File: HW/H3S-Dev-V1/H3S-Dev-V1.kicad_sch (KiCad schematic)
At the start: 38 parts, among them J1 USB_C_Receptacle_USB2.0_16P, J2 Conn_01x02_Socket, J3 Conn_Coaxial, Q1 DMP3099L, SW1 SW_Push, U1 Ai-Thinker-Ra-01, U2 LTC4054ES5-4.2, U3 USBLC6-2SC6, U4 ESP32-S3-WROOM-1, U5 SY8089AAAC, U6 L96-M33

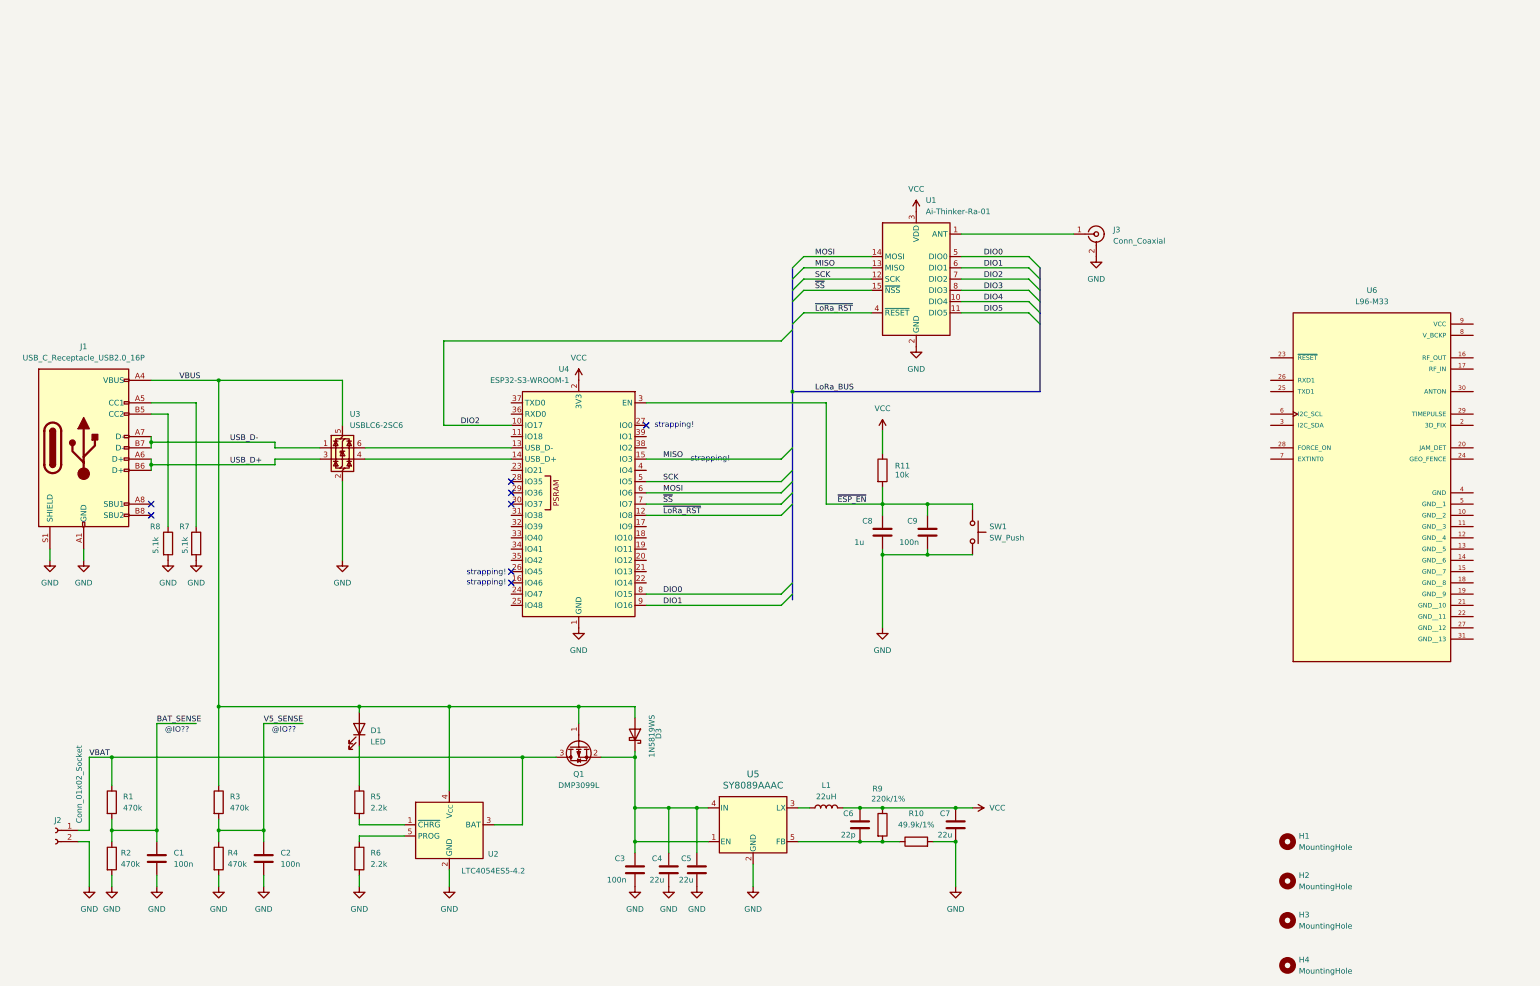
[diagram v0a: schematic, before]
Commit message: Some progress...
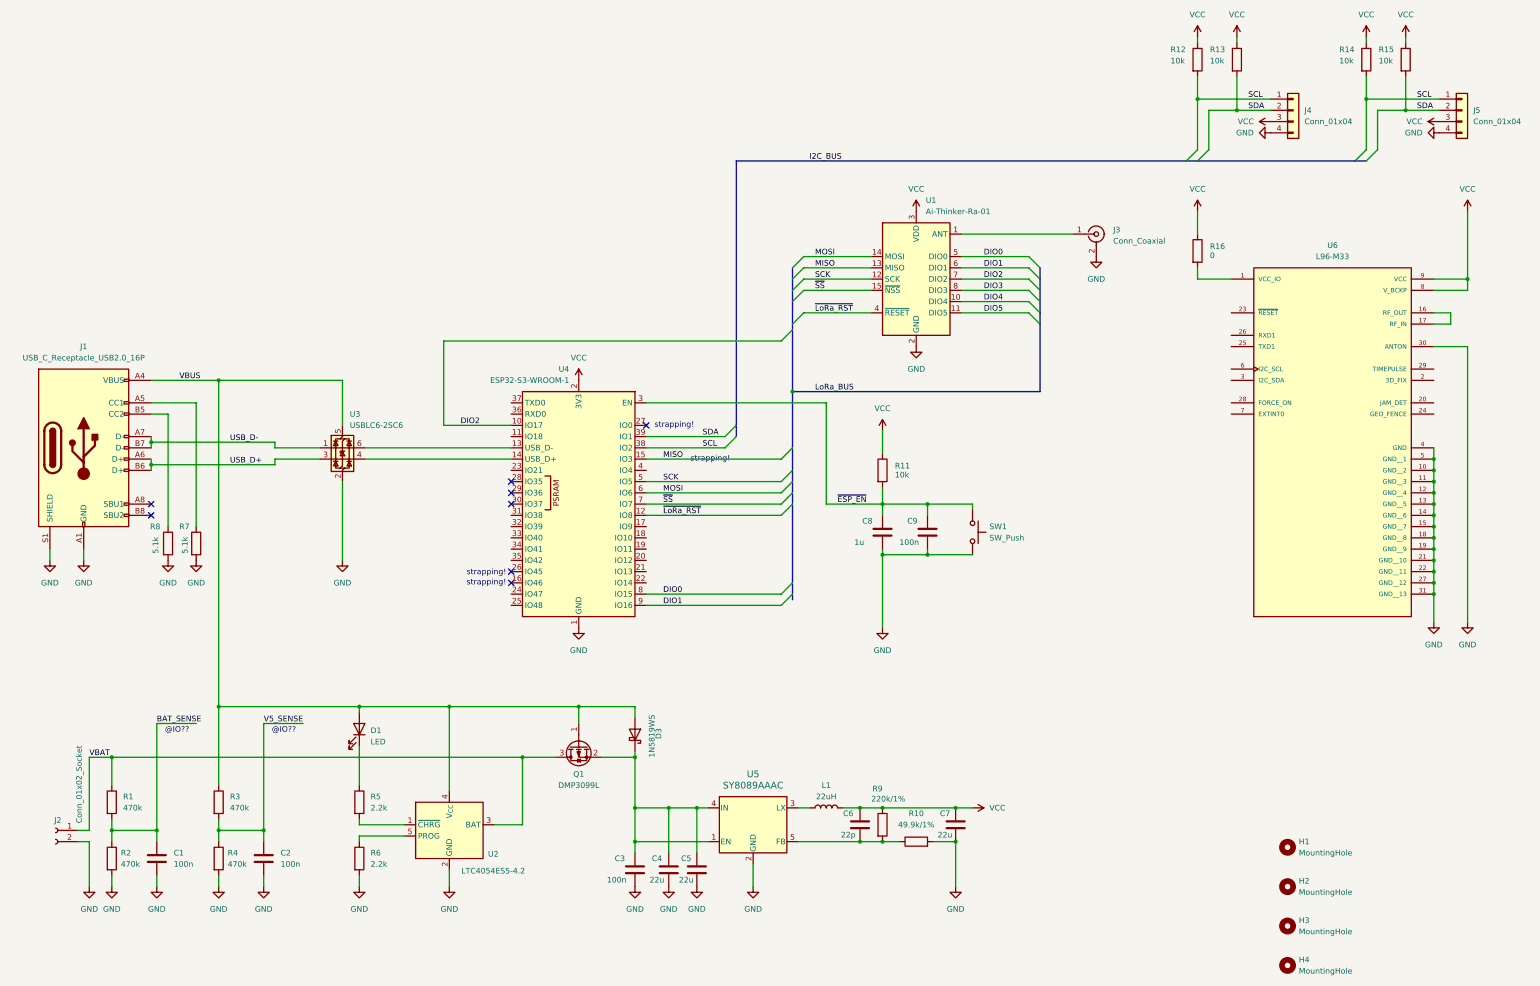
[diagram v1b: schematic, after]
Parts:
- added J4, J5: Conn_01x04, Connector:NS-Tech_Grove_1x04_P2mm_Vertical, symbol Connector_Generic:Conn_01x04
- added R12, R13, R14, R15: 10k, Resistor_SMD:R_0603_1608Metric, symbol Device:R
- added R16: 0, Resistor_SMD:R_0603_1608Metric, symbol Device:R
- U6: footprint L96_M33:XCVR_L96-M33 -> XCVR_L96-M33; DESCRIPTION L96 is a concurrent multi-GNSS receiver module with embedde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 -> (none)
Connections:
- net GND: now also U6.10 (GND__2), U6.11 (GND__3), U6.12 (GND__4), U6.13 (GND__5), U6.14 (GND__6), U6.15 (GND__7), U6.18 (GND__8), U6.19 (GND__9), U6.21 (GND__10), U6.22 (GND__11), U6.27 (GND__12), U6.30 (ANTON), U6.31 (GND__13), U6.4 (GND), U6.5 (GND__1), J4.4 (Pin_4), J5.4 (Pin_4)
- net VCC: now also U6.8 (V_BCKP), U6.9 (VCC), J4.3 (Pin_3), J5.3 (Pin_3), R12.1, R13.1, R14.1, R15.1, R16.1
- net SCL: now reaches U4.38 (IO2)
- net SCL: now also J4.1 (Pin_1), J5.1 (Pin_1), R12.2, R14.2
- net SDA: now reaches U4.39 (IO1)
- net SDA: now also J4.2 (Pin_2), J5.2 (Pin_2), R13.2, R15.2
- net at U6.16 (RF_OUT): now also U6.17 (RF_IN)
- new net: R16.2, U6.1 (VCC_IO)
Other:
- moved on the sheet: H1, H2, H3
